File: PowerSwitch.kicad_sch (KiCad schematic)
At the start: 16 parts, among them U401 BTT6010

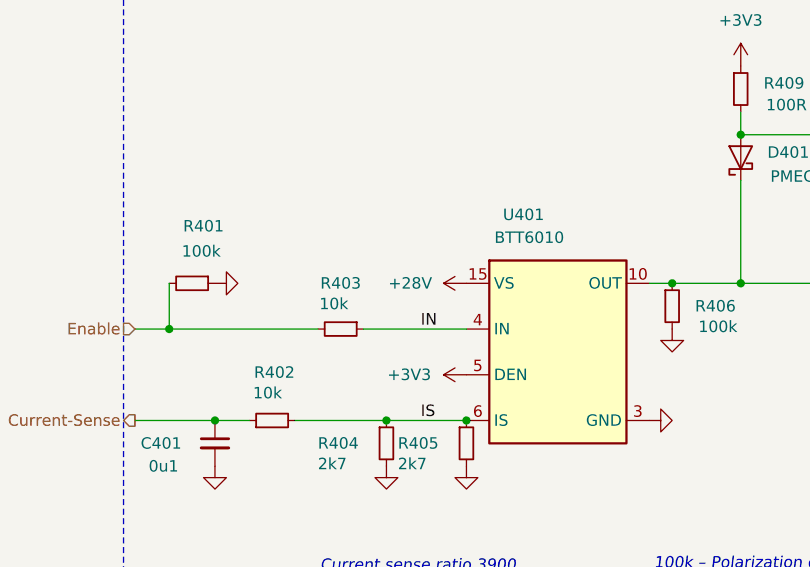
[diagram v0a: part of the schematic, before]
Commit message: Refresh
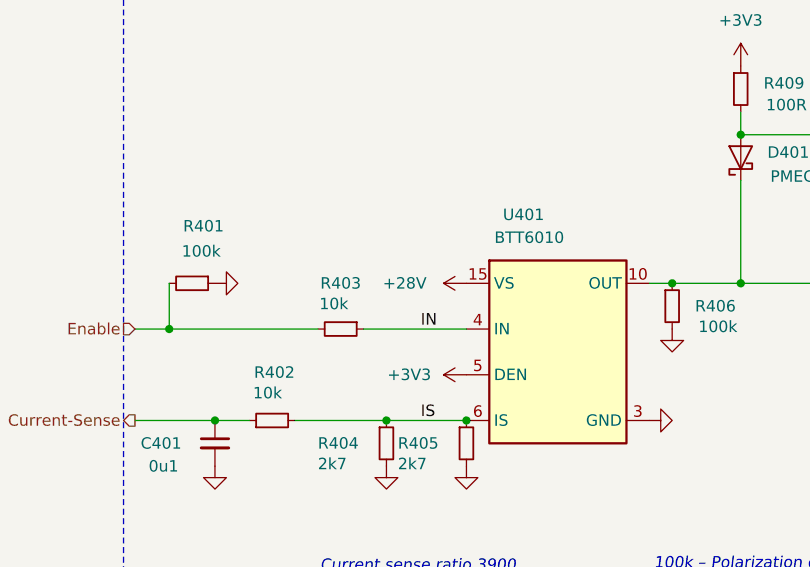
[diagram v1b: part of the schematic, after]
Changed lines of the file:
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@@
 		(in_pos_files no)
 		(dnp no)
-		(property "Reference" "#PWR0409"
+		(property "Reference" "#PWR409"
 			(at 166.37 48.26 0)
 			(hide yes)
@@
 				(font
 					(size 1.27 1.27)
+					(color 255 92 187 1)
 				)
 			)
@@
 			(project "drum"
 				(path "/6c8448b4-b04d-47e1-934e-e40cbe27a7be/ba748654-beb9-4861-aa35-c19e08caaf2e"
-					(reference "#PWR0409")
+					(reference "#PWR409")
 					(unit 1)
 				)
@@
 		(in_pos_files yes)
 		(dnp no)
-		(property "Reference" "#PWR0414"
+		(property "Reference" "#PWR414"
 			(at 191.77 63.5 0)
 			(hide yes)
@@
 			(project "drum"
 				(path "/6c8448b4-b04d-47e1-934e-e40cbe27a7be/ba748654-beb9-4861-aa35-c19e08caaf2e"
-					(reference "#PWR0414")
+					(reference "#PWR414")
 					(unit 1)
 				)
@@
 		(in_pos_files yes)
 		(dnp no)
-		(property "Reference" "#PWR0403"
+		(property "Reference" "#PWR403"
 			(at 127 143.51 0)
 			(hide yes)
@@
 			(project "drum"
 				(path "/6c8448b4-b04d-47e1-934e-e40cbe27a7be/ba748654-beb9-4861-aa35-c19e08caaf2e"
-					(reference "#PWR0403")
+					(reference "#PWR403")
 					(unit 1)
 				)
@@
 		(in_pos_files yes)
 		(dnp no)
-		(property "Reference" "#PWR0412"
+		(property "Reference" "#PWR412"
 			(at 184.15 128.27 0)
 			(hide yes)
@@
 			(project "drum"
 				(path "/6c8448b4-b04d-47e1-934e-e40cbe27a7be/ba748654-beb9-4861-aa35-c19e08caaf2e"
-					(reference "#PWR0412")
+					(reference "#PWR412")
 					(unit 1)
 				)
@@
 		(in_pos_files yes)
 		(dnp no)
-		(property "Reference" "#PWR0401"
+		(property "Reference" "#PWR401"
 			(at 114.3 116.84 0)
 			(hide yes)
@@
 			(project "drum"
 				(path "/6c8448b4-b04d-47e1-934e-e40cbe27a7be/ba748654-beb9-4861-aa35-c19e08caaf2e"
-					(reference "#PWR0401")
+					(reference "#PWR401")
 					(unit 1)
 				)
@@
 		(in_pos_files yes)
 		(dnp no)
-		(property "Reference" "#PWR0413"
+		(property "Reference" "#PWR413"
 			(at 186.69 111.76 0)
 			(hide yes)
@@
 			(project "drum"
 				(path "/6c8448b4-b04d-47e1-934e-e40cbe27a7be/ba748654-beb9-4861-aa35-c19e08caaf2e"
-					(reference "#PWR0413")
+					(reference "#PWR413")
 					(unit 1)
 				)
@@
 		(in_pos_files yes)
 		(dnp no)
-		(property "Reference" "#PWR0411"
+		(property "Reference" "#PWR411"
 			(at 166.37 96.52 0)
 			(hide yes)
@@
 				(font
 					(size 1.27 1.27)
+					(color 255 92 187 1)
 				)
 			)
@@
 			(project "drum"
 				(path "/6c8448b4-b04d-47e1-934e-e40cbe27a7be/ba748654-beb9-4861-aa35-c19e08caaf2e"
-					(reference "#PWR0411")
+					(reference "#PWR411")
 					(unit 1)
 				)
@@
 		(in_pos_files yes)
 		(dnp no)
-		(property "Reference" "#PWR0407"
+		(property "Reference" "#PWR407"
 			(at 162.56 132.08 0)
 			(hide yes)
@@
 			(project "drum"
 				(path "/6c8448b4-b04d-47e1-934e-e40cbe27a7be/ba748654-beb9-4861-aa35-c19e08caaf2e"
-					(reference "#PWR0407")
+					(reference "#PWR407")
 					(unit 1)
 				)
@@
 		(in_pos_files no)
 		(dnp no)
-		(fields_autoplaced yes)
-		(property "Reference" "#PWR0404"
+		(property "Reference" "#PWR404"
 			(at 139.7 116.84 0)
 			(hide yes)
@@
 		)
 		(property "Value" "+28V"
-			(at 132.08 116.8399 90)
+			(at 129.032 116.8399 90)
 			(show_name no)
 			(do_not_autoplace no)
@@
 				(font
 					(size 1.27 1.27)
+					(color 255 92 187 1)
 				)
-				(justify left)
 			)
 		)
@@
 			(project "drum"
 				(path "/6c8448b4-b04d-47e1-934e-e40cbe27a7be/ba748654-beb9-4861-aa35-c19e08caaf2e"
-					(reference "#PWR0404")
+					(reference "#PWR404")
 					(unit 1)
 				)
@@
 		(in_pos_files yes)
 		(dnp no)
-		(property "Reference" "#PWR0406"
+		(property "Reference" "#PWR406"
 			(at 135.89 143.51 0)
 			(hide yes)
@@
 			(project "drum"
 				(path "/6c8448b4-b04d-47e1-934e-e40cbe27a7be/ba748654-beb9-4861-aa35-c19e08caaf2e"
-					(reference "#PWR0406")
+					(reference "#PWR406")
 					(unit 1)
 				)
@@
 		(in_pos_files yes)
 		(dnp no)
-		(property "Reference" "#PWR0410"
+		(property "Reference" "#PWR410"
 			(at 166.37 63.5 0)
 			(hide yes)
@@
 			(project "drum"
 				(path "/6c8448b4-b04d-47e1-934e-e40cbe27a7be/ba748654-beb9-4861-aa35-c19e08caaf2e"
-					(reference "#PWR0410")
+					(reference "#PWR410")
 					(unit 1)
 				)
@@
 		(in_pos_files yes)
 		(dnp no)
-		(property "Reference" "#PWR0408"
+		(property "Reference" "#PWR408"
 			(at 158.75 128.27 0)
 			(hide yes)
@@
 			(project "drum"
 				(path "/6c8448b4-b04d-47e1-934e-e40cbe27a7be/ba748654-beb9-4861-aa35-c19e08caaf2e"
-					(reference "#PWR0408")
+					(reference "#PWR408")
 					(unit 1)
 				)
@@
 		(in_pos_files yes)
 		(dnp no)
-		(property "Reference" "#PWR0402"
+		(property "Reference" "#PWR402"
 			(at 107.95 143.51 0)
 			(hide yes)
@@
 			(project "drum"
 				(path "/6c8448b4-b04d-47e1-934e-e40cbe27a7be/ba748654-beb9-4861-aa35-c19e08caaf2e"
-					(reference "#PWR0402")
+					(reference "#PWR402")
 					(unit 1)
 				)
@@
 		(in_pos_files yes)
 		(dnp no)
-		(property "Reference" "#PWR0405"
+		(property "Reference" "#PWR405"
 			(at 139.7 127 0)
 			(hide yes)
@@
 				(font
 					(size 1.27 1.27)
+					(color 255 92 187 1)
 				)
 			)
@@
 			(project "drum"
 				(path "/6c8448b4-b04d-47e1-934e-e40cbe27a7be/ba748654-beb9-4861-aa35-c19e08caaf2e"
-					(reference "#PWR0405")
+					(reference "#PWR405")
 					(unit 1)
 				)
